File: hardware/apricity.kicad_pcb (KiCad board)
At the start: 2 copper layers, 71.2 x 71.2 mm, 26 parts, among them J1 USB_C_Receptacle_USB2.0, U1 ESP-WROOM-02D, U2 X

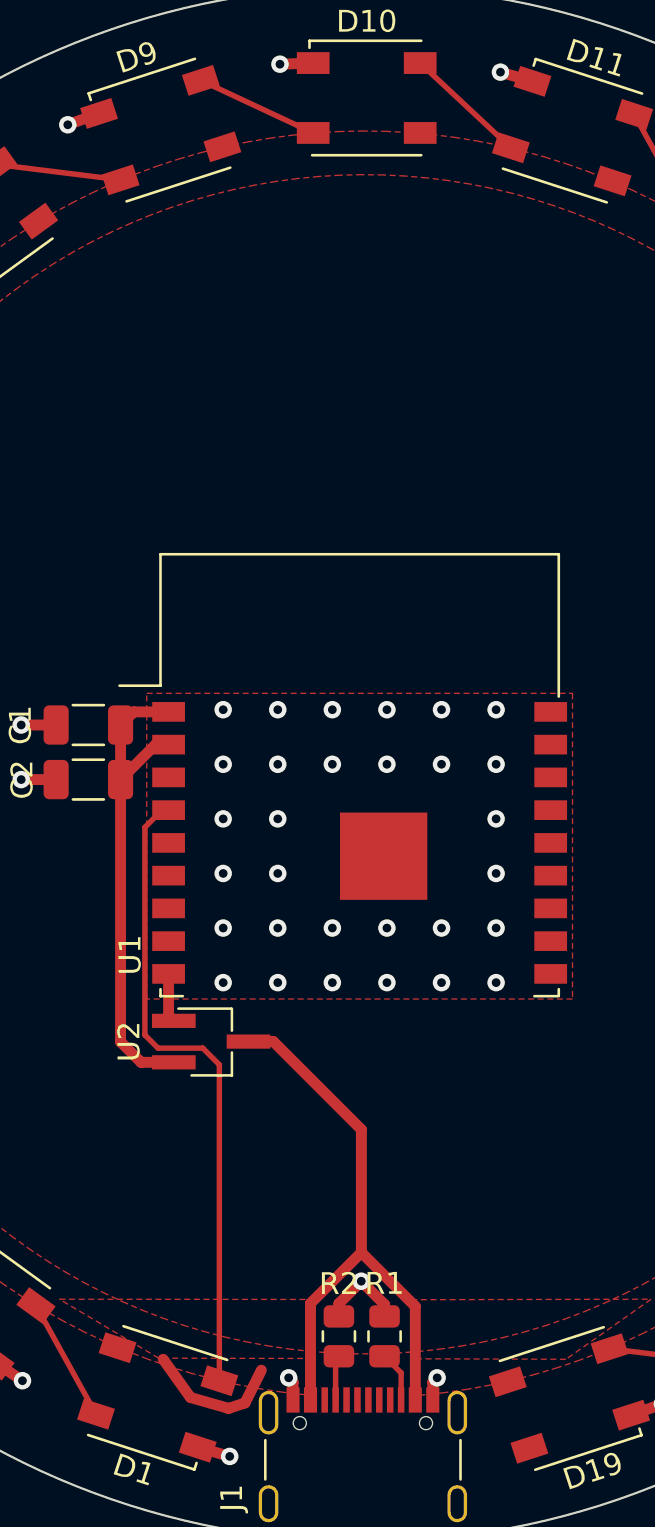
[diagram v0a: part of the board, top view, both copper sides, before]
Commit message: remove loops
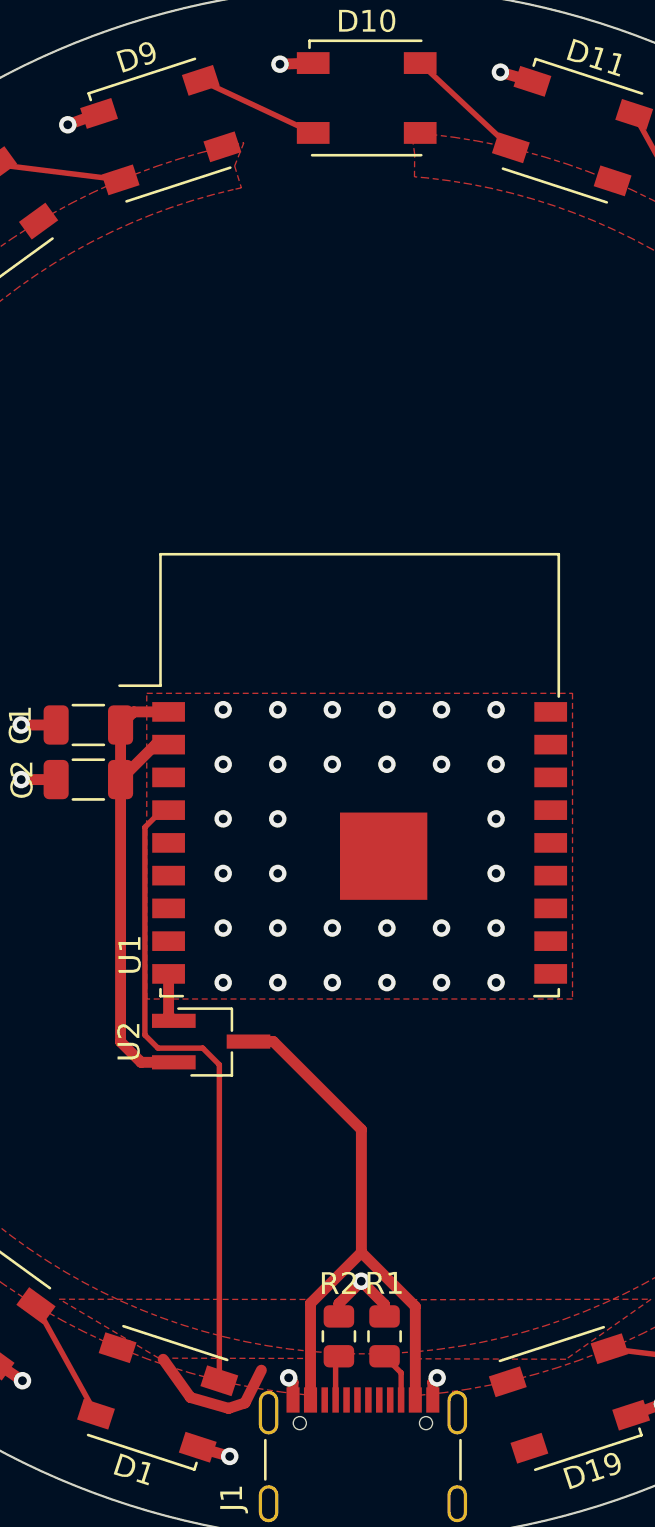
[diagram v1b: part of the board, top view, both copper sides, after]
